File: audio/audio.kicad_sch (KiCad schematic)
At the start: 0 parts

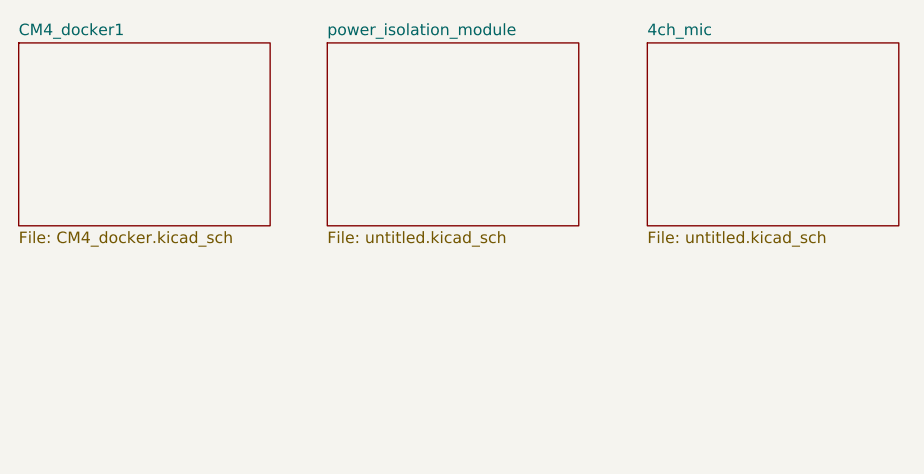
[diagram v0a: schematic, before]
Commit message: .
.
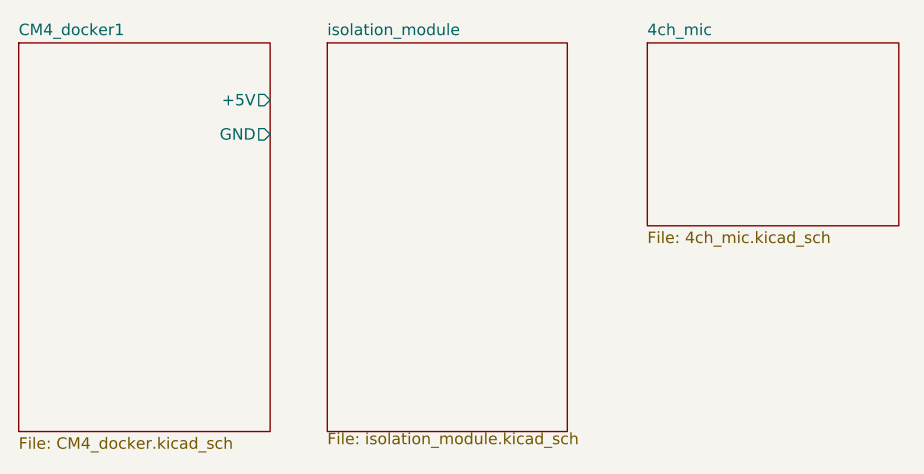
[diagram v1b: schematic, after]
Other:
- sheet power_isolation_module renamed isolation_module
- sheet 4ch_mic: file untitled.kicad_sch -> 4ch_mic.kicad_sch
- sheet CM4_docker1 ports: added +5V, GND; removed none
- sheet isolation_module: file untitled.kicad_sch -> isolation_module.kicad_sch
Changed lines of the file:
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@@
 (kicad_sch (version 20211123) (generator eeschema)
   (paper "A4")
-  (sheet (at 63.5 26.67) (size 27.94 20.32) (fields_autoplaced)
+  (sheet (at 63.5 26.67) (size 26.67 43.18) (fields_autoplaced)
     (stroke (width 0.1524) (type solid) (color 0 0 0 0))
     (fill (color 0 0 0 0.0000))
-    (property "Sheet name" "power_isolation_module" (id 0) (at 63.5 25.9584 0)
+    (property "Sheet name" "isolation_module" (id 0) (at 63.5 25.9584 0)
       (effects (font (size 1.27 1.27)) (justify left bottom))
     )
-    (property "Sheet file" "untitled.kicad_sch" (id 1) (at 63.5 47.5746 0)
-      (effects (font (size 1.27 1.27)) (justify left top))
+    (property "Sheet file" "isolation_module.kicad_sch" (id 1) (at 63.5 69.9266 0)
+      (effects (font (size 0 0)) (justify left top))
     )
   )
@@
       (effects (font (size 1.27 1.27)) (justify left bottom))
     )
-    (property "Sheet file" "untitled.kicad_sch" (id 1) (at 99.06 47.5746 0)
+    (property "Sheet file" "4ch_mic.kicad_sch" (id 1) (at 99.06 47.5746 0)
       (effects (font (size 1.27 1.27)) (justify left top))
     )
   )
-  (sheet (at 29.21 26.67) (size 27.94 20.32) (fields_autoplaced)
+  (sheet (at 29.21 26.67) (size 27.94 43.18) (fields_autoplaced)
     (stroke (width 0.1524) (type solid) (color 0 0 0 0))
     (fill (color 0 0 0 0.0000))
@@
       (effects (font (size 1.27 1.27)) (justify left bottom))
     )
-    (property "Sheet file" "CM4_docker.kicad_sch" (id 1) (at 29.21 47.5746 0)
+    (property "Sheet file" "CM4_docker.kicad_sch" (id 1) (at 29.21 70.4346 0)
       (effects (font (size 1.27 1.27)) (justify left top))
     )
+    (pin "+5V" output (at 57.15 33.02 0)
+      (effects (font (size 1.27 1.27)) (justify right))
+    )
+    (pin "GND" output (at 57.15 36.83 0)
+      (effects (font (size 1.27 1.27)) (justify right))
+    )
   )
